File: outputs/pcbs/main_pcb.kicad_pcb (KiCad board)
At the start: 2 copper layers, 166.5 x 128.8 mm, 89 parts

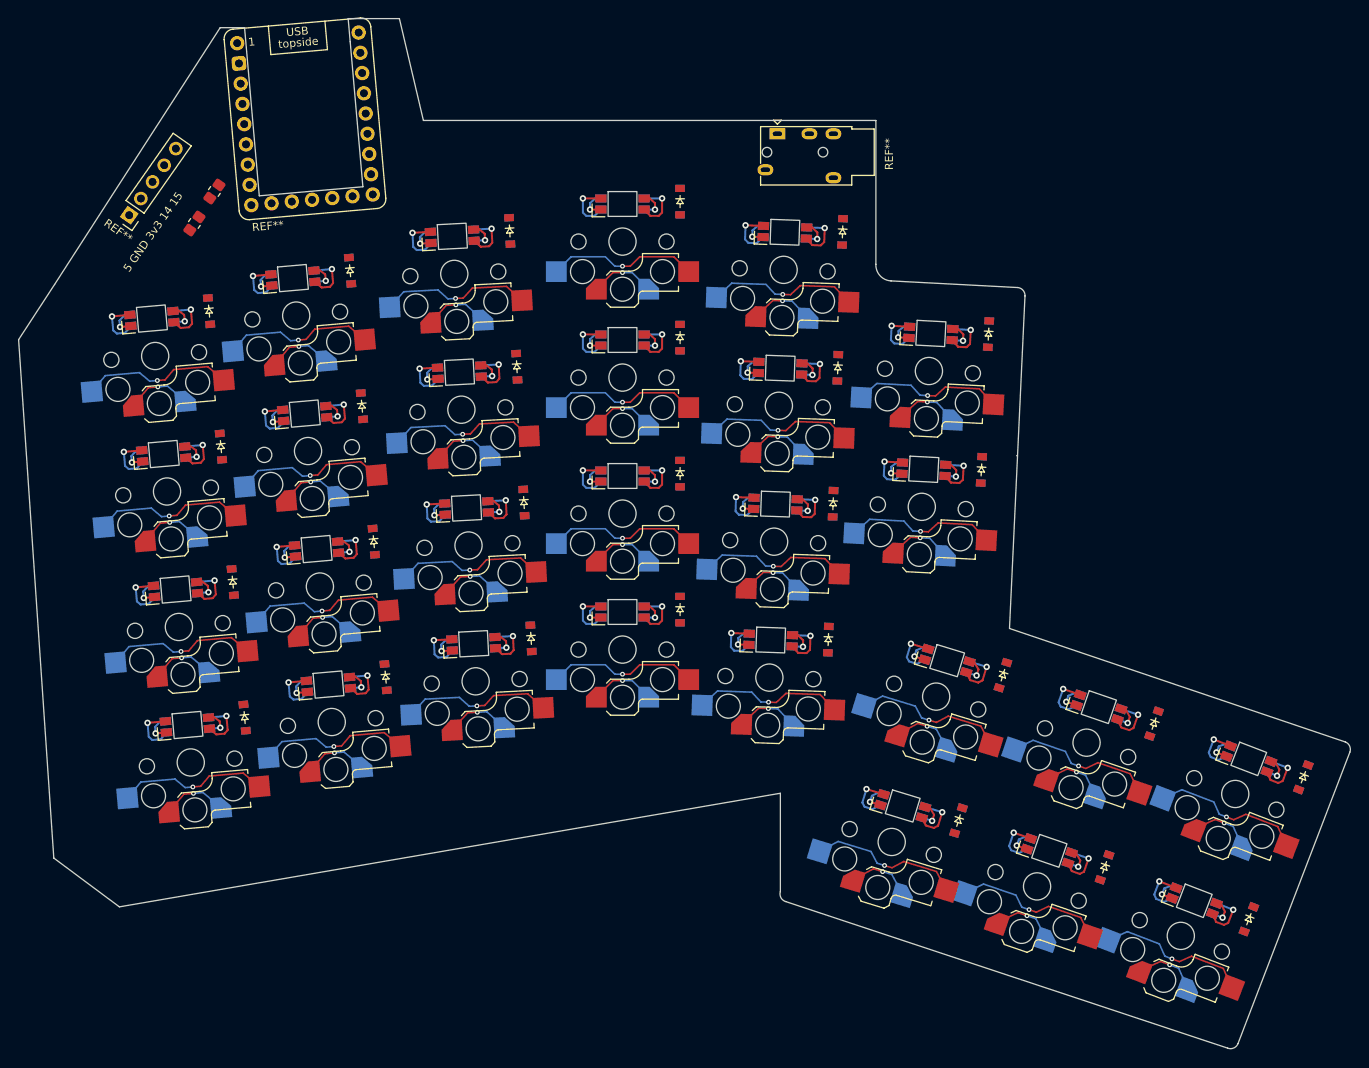
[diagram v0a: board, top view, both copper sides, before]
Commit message: routing1
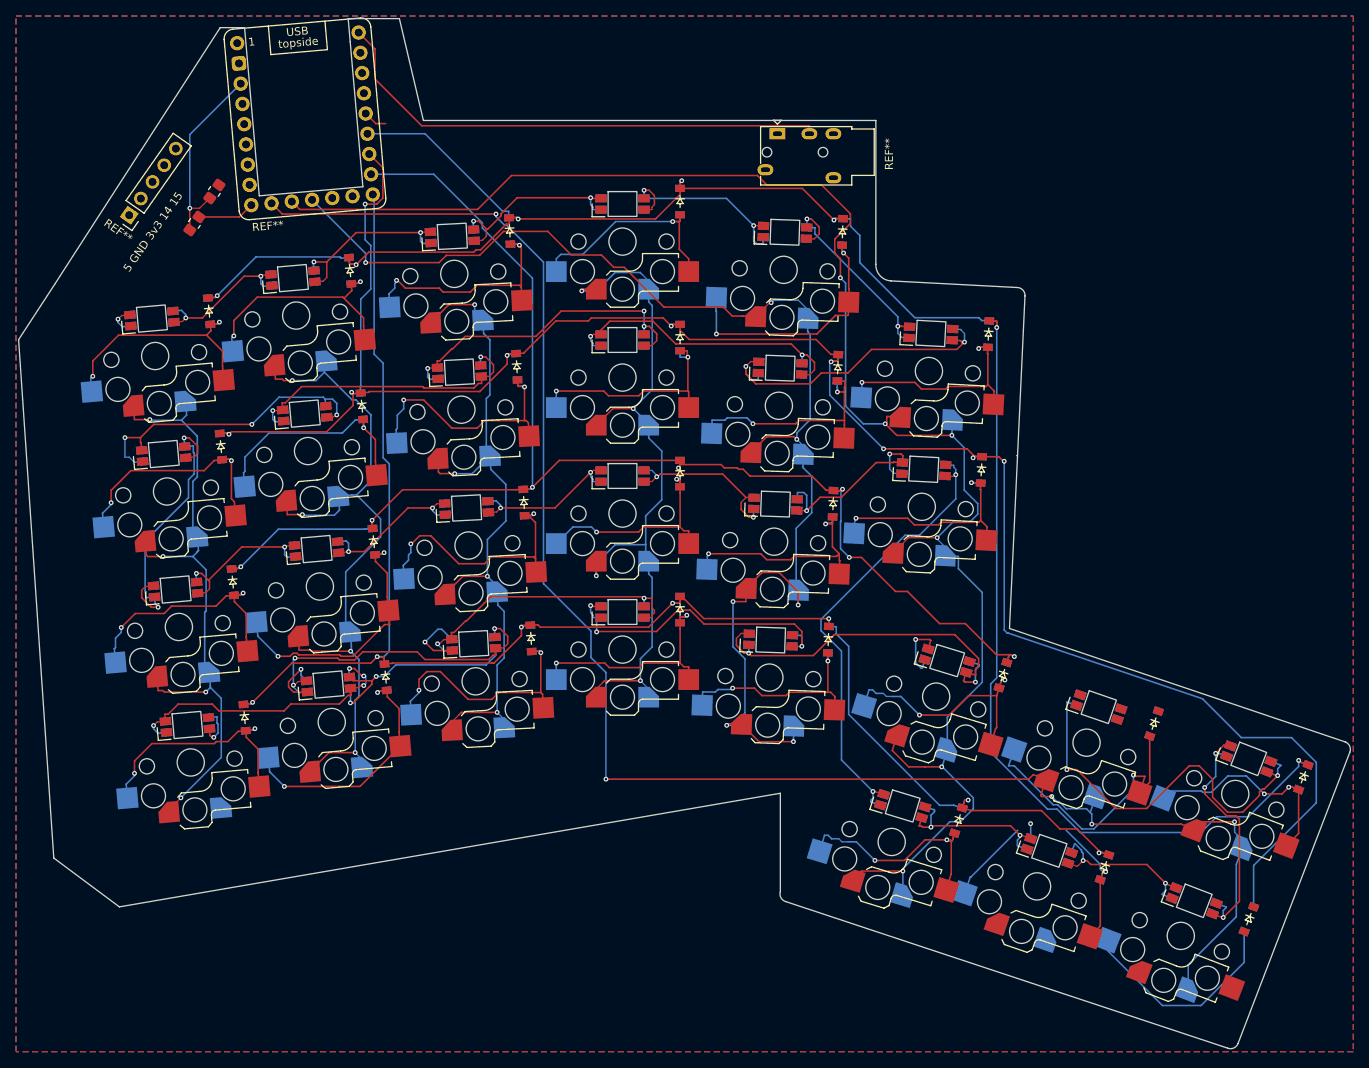
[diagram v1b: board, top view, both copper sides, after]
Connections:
- REF** pad 15: R_3 -> R_0
- REF** pad 16: R_2 -> R_1
- REF** pad 17: R_1 -> R_2
- REF** pad 18: R_0 -> R_3
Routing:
- net R_0: track 0.00 -> 251.5 mm, vias 0 -> 7
- net R_1: track 0.00 -> 246.1 mm, vias 0 -> 9
- net R_3: track 0.00 -> 205.4 mm, vias 0 -> 7
- net t_2: track 33.1 -> 215.8 mm, vias 4 -> 5
- net K_5: track 33.1 -> 214.3 mm, vias 4 -> 6
- net R_2: track 0.00 -> 180.2 mm, vias 0 -> 7
- net K_4: track 33.1 -> 161.4 mm, vias 4 -> 7
- net GND: track 105.1 -> 17.5 mm, vias 28 -> 3
- net VCC: track 105.1 -> 26.6 mm, vias 28 -> 2
- net cross_board: track 0.00 -> 64.4 mm
- net K_1: track 33.1 -> 94.5 mm
- net K_3: track 33.1 -> 91.5 mm
- net K_2: track 33.1 -> 89.4 mm
- net K_0: track 33.1 -> 81.4 mm
- net D17: track 13.5 -> 58.1 mm
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- added copper zone on B.Cu, net GND
- added copper zone on F.Cu, net VCC
